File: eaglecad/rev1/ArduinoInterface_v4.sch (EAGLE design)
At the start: 49 parts, among them IC1 74LS00N, IC11 74LS20N, IC2 74LS373N, IC3 74LS30N, IC4 74LS244N, IC5 74S74N, IC6 74LS139N, IC7 74LS155N, IC9 7805TV, J1 Connector, J2 TEENSY_CONN, J3 GLUE_CONN

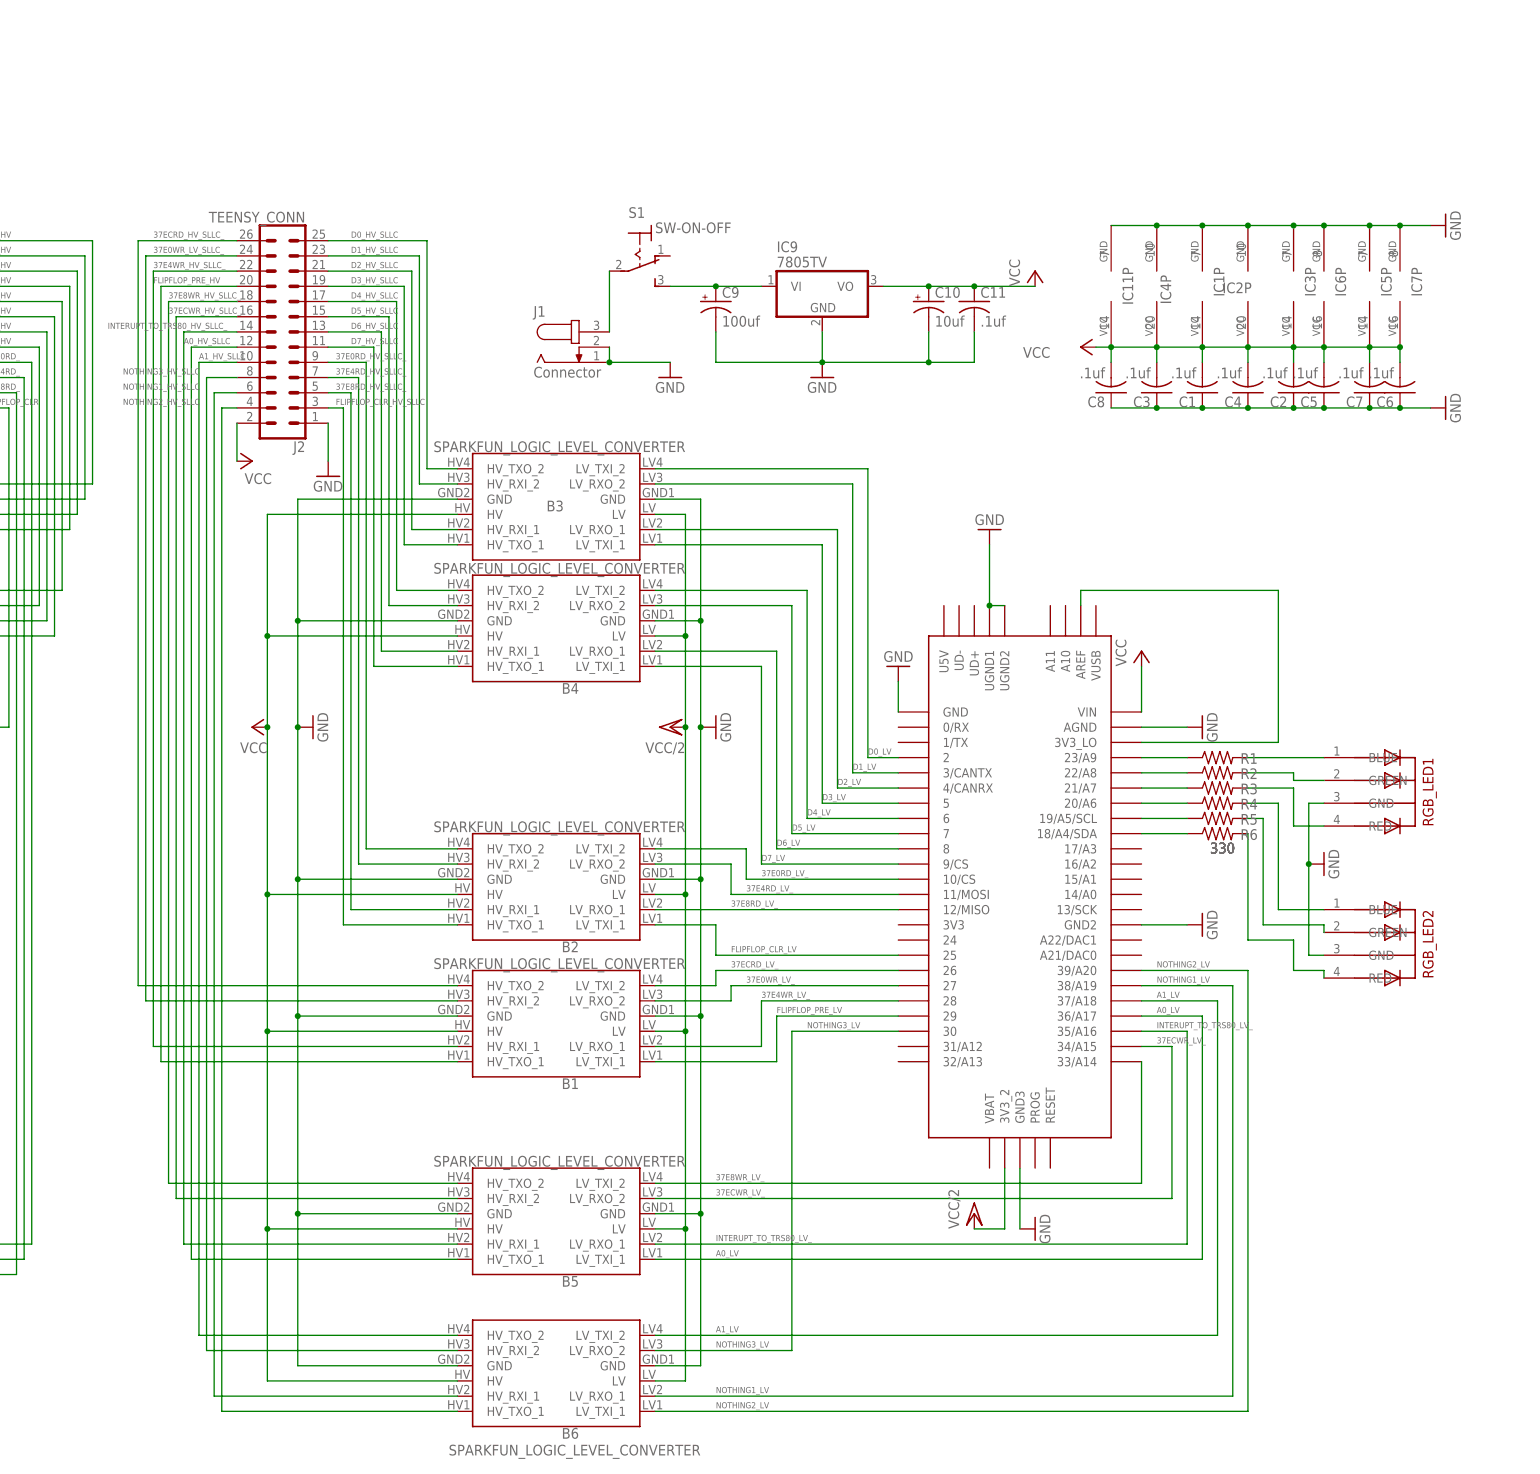
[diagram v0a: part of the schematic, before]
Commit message: updates to v4 schematic
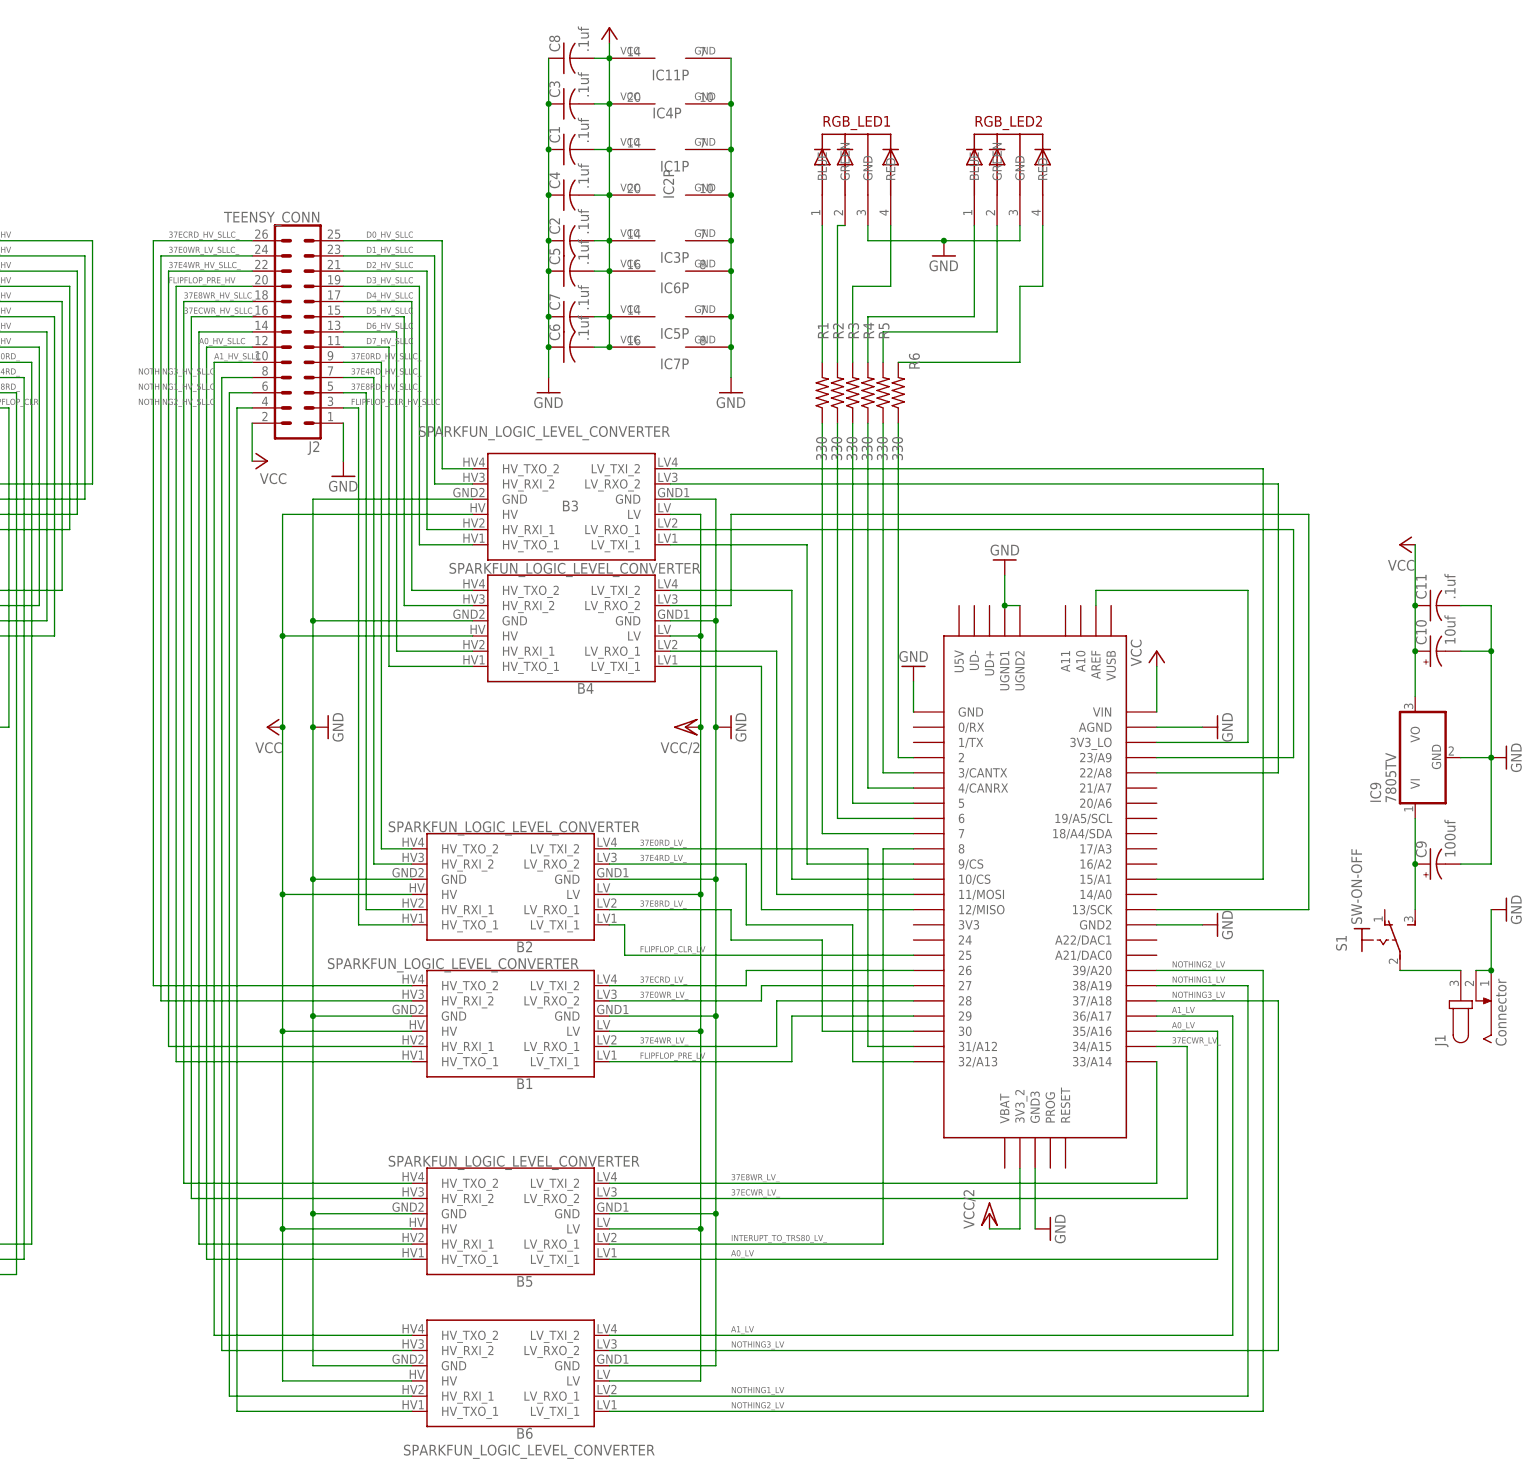
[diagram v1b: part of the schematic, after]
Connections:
- removed net N$16: R4.1, U$2.20/A6
- removed net N$17: R5.1, U$2.19/A5/SCL
- removed net N$18: R6.1, U$2.18/A4/SDA
- removed net N$9: R3.1, U$2.21/A7
- new net N$3: R6.1, U$2.2
- new net N$4: R5.1, U$2.3/CANTX
- new net N$7: R2.1, U$2.6
- new net N$8: R1.1, U$2.7
- net 37E0RD_LV_: now also U$2.31/A12; no longer U$2.10/CS
- net 37E4RD_LV_: now also U$2.32/A13; no longer U$2.11/MOSI
- net 37E8RD_LV_: now also U$2.30; no longer U$2.12/MISO
- net A0_LV: now also U$2.35/A16; no longer U$2.36/A17
- net A1_LV: now also U$2.36/A17; no longer U$2.37/A18
- net D0_LV: now also U$2.15/A1; no longer U$2.2
- net D1_LV: now also U$2.22/A8; no longer U$2.3/CANTX
- net D2_LV: now also U$2.23/A9; no longer U$2.4/CANRX
- net D3_LV: now also U$2.9/CS; no longer U$2.5
- net D4_LV: now also U$2.10/CS; no longer U$2.6
- net D5_LV: now also U$2.13/SCK; no longer U$2.7
- net D6_LV: now also U$2.11/MOSI; no longer U$2.8
- net D7_LV: now also U$2.12/MISO; no longer U$2.9/CS
- net INTERUPT_TO_TRS80_LV_: now also U$2.8; no longer U$2.35/A16
- net N$5: now also R4.1, U$2.4/CANRX; no longer R1.1, U$2.23/A9
- net N$6: now also R3.1, U$2.5; no longer R2.1, U$2.22/A8
- net NOTHING3_LV: now also U$2.37/A18; no longer U$2.30
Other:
- moved on the sheet: B1, B2, B3, B4, B5, B6, C1, C10, C11, C2, C3, C4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
